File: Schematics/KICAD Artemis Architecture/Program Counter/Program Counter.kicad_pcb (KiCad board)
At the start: 4 copper layers, 62.6 x 31.6 mm, 26 parts, among them J1 Bus, J2 Power, J3 Control, Q1 2N3904, U1 74LS161, U2 74LS161, U3 74LS245

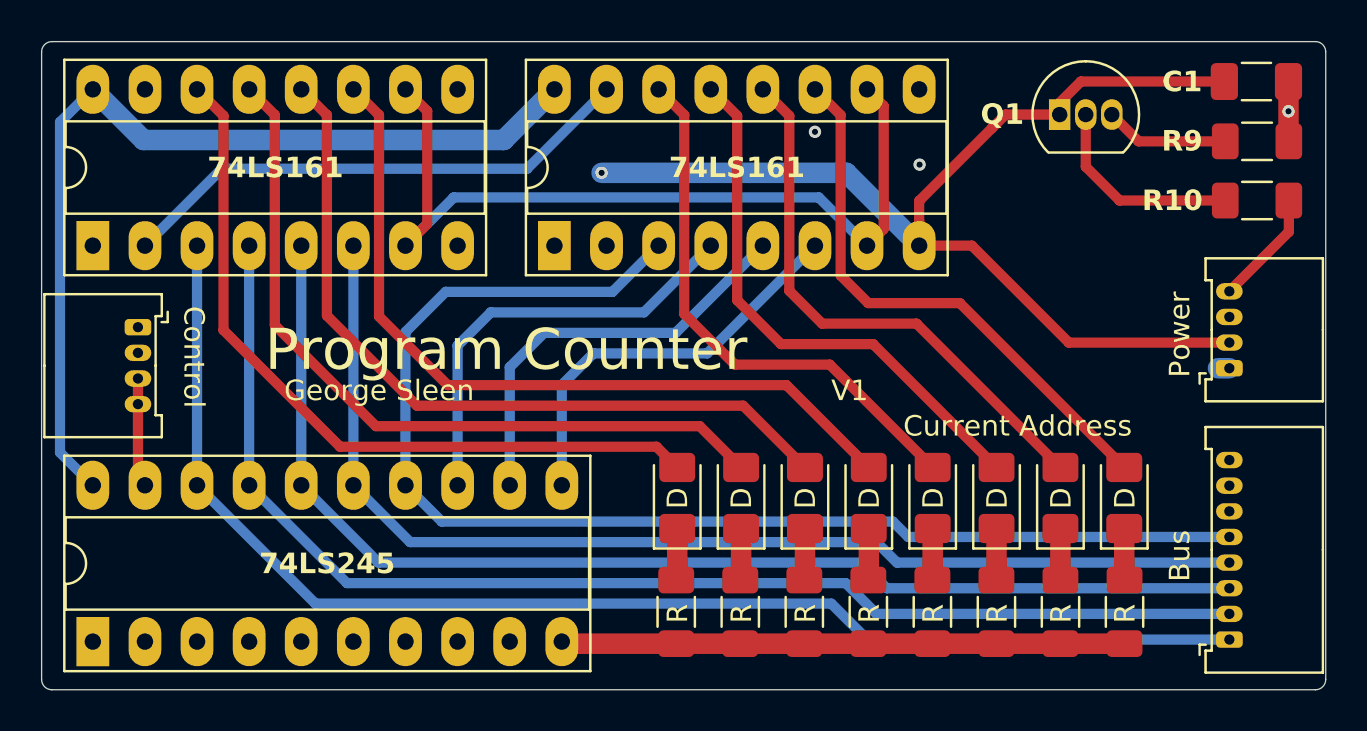
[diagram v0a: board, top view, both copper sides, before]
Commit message: Program Memory
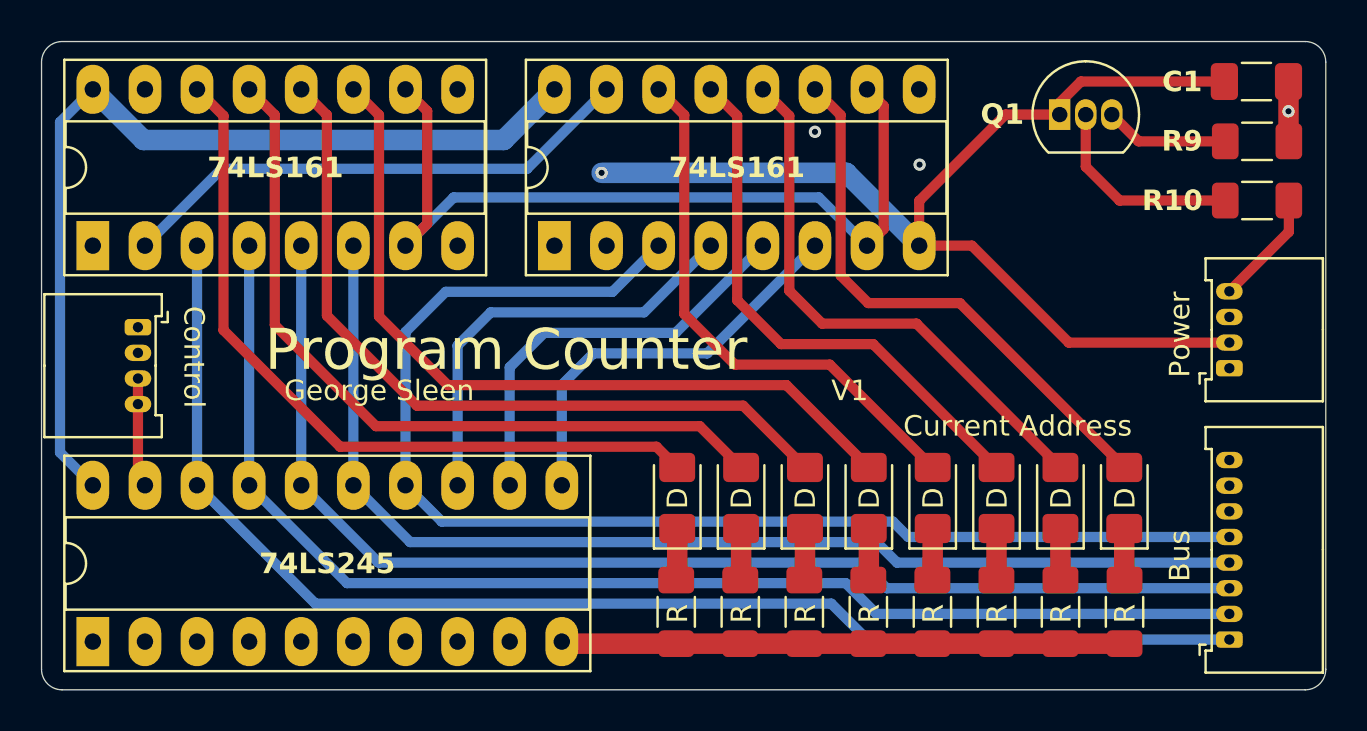
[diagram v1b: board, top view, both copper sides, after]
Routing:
- net VCC: track 154.8 -> 153.3 mm
- net GNDREF: track 82.6 -> 81.3 mm
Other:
- outline, holes or cut-outs redrawn
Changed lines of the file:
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@@
 		)
 	)
-	(gr_line
-		(start 102.203553 61.003553)
-		(end 163.796447 61.003553)
+	(gr_arc
+		(start 101.7 62)
+		(mid 101.992893 61.292893)
+		(end 102.7 61)
 		(stroke
 			(width 0.05)
@@
 		(layer "Edge.Cuts")
 	)
-	(gr_arc
-		(start 101.703553 61.503553)
-		(mid 101.85 61.15)
-		(end 102.203553 61.003553)
+	(gr_line
+		(start 164.3 62)
+		(end 164.3 91.6)
 		(stroke
 			(width 0.05)
@@
 	)
 	(gr_arc
-		(start 163.796447 61.003553)
-		(mid 164.15 61.15)
-		(end 164.296447 61.503553)
+		(start 164.3 91.6)
+		(mid 164.007107 92.307107)
+		(end 163.3 92.6)
 		(stroke
 			(width 0.05)
@@
 		(layer "Edge.Cuts")
 	)
-	(gr_arc
-		(start 102.203553 92.596447)
-		(mid 101.85 92.45)
-		(end 101.703553 92.096447)
+	(gr_line
+		(start 101.7 91.6)
+		(end 101.7 62)
 		(stroke
 			(width 0.05)
@@
 	)
 	(gr_line
-		(start 163.796447 92.596447)
-		(end 102.203553 92.596447)
+		(start 163.3 92.6)
+		(end 102.7 92.6)
 		(stroke
 			(width 0.05)
@@
 		(layer "Edge.Cuts")
 	)
-	(gr_line
-		(start 164.296447 61.503553)
-		(end 164.296447 92.096447)
+	(gr_arc
+		(start 102.7 92.6)
+		(mid 101.992893 92.307107)
+		(end 101.7 91.6)
 		(stroke
 			(width 0.05)
@@
 	)
 	(gr_line
-		(start 101.703553 92.096447)
-		(end 101.703553 61.503553)
+		(start 102.7 61)
+		(end 163.3 61)
 		(stroke
 			(width 0.05)
@@
 	)
 	(gr_arc
-		(start 164.296447 92.096447)
-		(mid 164.15 92.45)
-		(end 163.796447 92.596447)
+		(start 163.3 61)
+		(mid 164.007107 61.292893)
+		(end 164.3 62)
 		(stroke
 			(width 0.05)
@@
 	)
 	(segment
-		(start 144.48 70.95)
-		(end 144.48 69.72)
-		(width 0.5)
-		(layer "F.Cu")
-		(net 2)
-	)
-	(segment
 		(start 135.758984 90.35)
 		(end 138.88082 90.35)
@@
 	)
 	(segment
-		(start 148.025 65.225)
-		(end 144.48 68.77)
+		(start 144.48 68.77)
+		(end 148.69 64.56)
 		(width 0.5)
 		(layer "F.Cu")
@@
 		(start 152.36 62.95)
 		(end 159.3575 62.95)
-		(width 0.5)
-		(layer "F.Cu")
-		(net 2)
-	)
-	(segment
-		(start 148.025 65.225)
-		(end 148.69 64.56)
 		(width 0.5)
 		(layer "F.Cu")
@@
 	)
 	(segment
-		(start 104.2 63.33)
-		(end 103.92 63.33)
-		(width 1)
-		(layer "In2.Cu")
-		(net 11)
-	)
-	(segment
 		(start 102.6 64.93)
 		(end 104.2 63.33)
@@
 		(layer "B.Cu")
 		(net 11)
-	)
-	(segment
-		(start 126.7 63.33)
-		(end 126.7 63.95)
-		(width 1)
-		(layer "B.Cu")
-		(net 11)
-	)
-	(segment
-		(start 159.044365 76.925)
-		(end 159.6 76.925)
-		(width 1)
-		(layer "B.Cu")
-		(net 11)
